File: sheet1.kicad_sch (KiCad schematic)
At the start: 18 parts, among them U1 8284A, U2 LS245, U22 74LS04, U25 8259A, U3 8088, U4 8087, U5 LS373, U6 LS244, U7 LS373, U8 8288, Y1 14.31818MHz

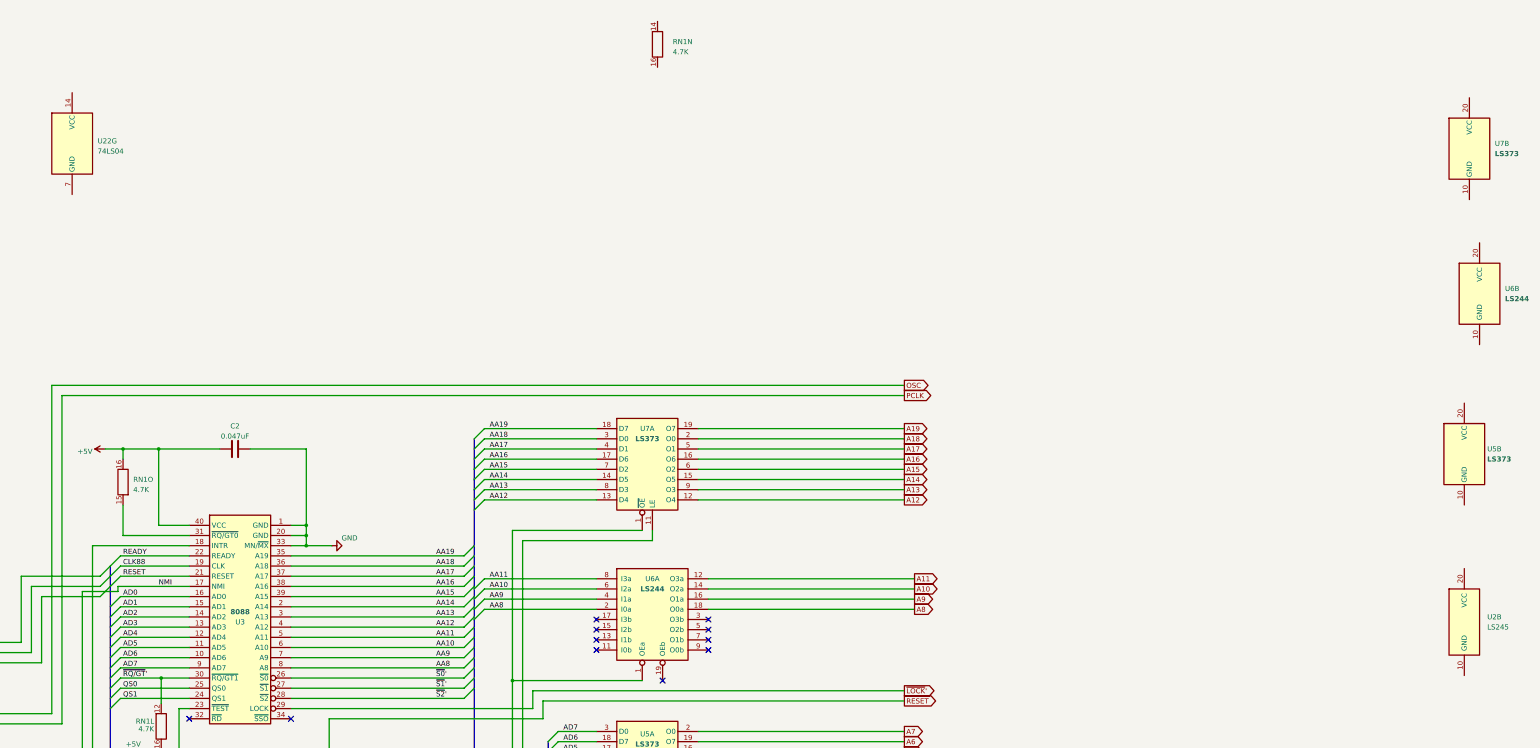
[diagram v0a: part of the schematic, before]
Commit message: Sheet 3 finished
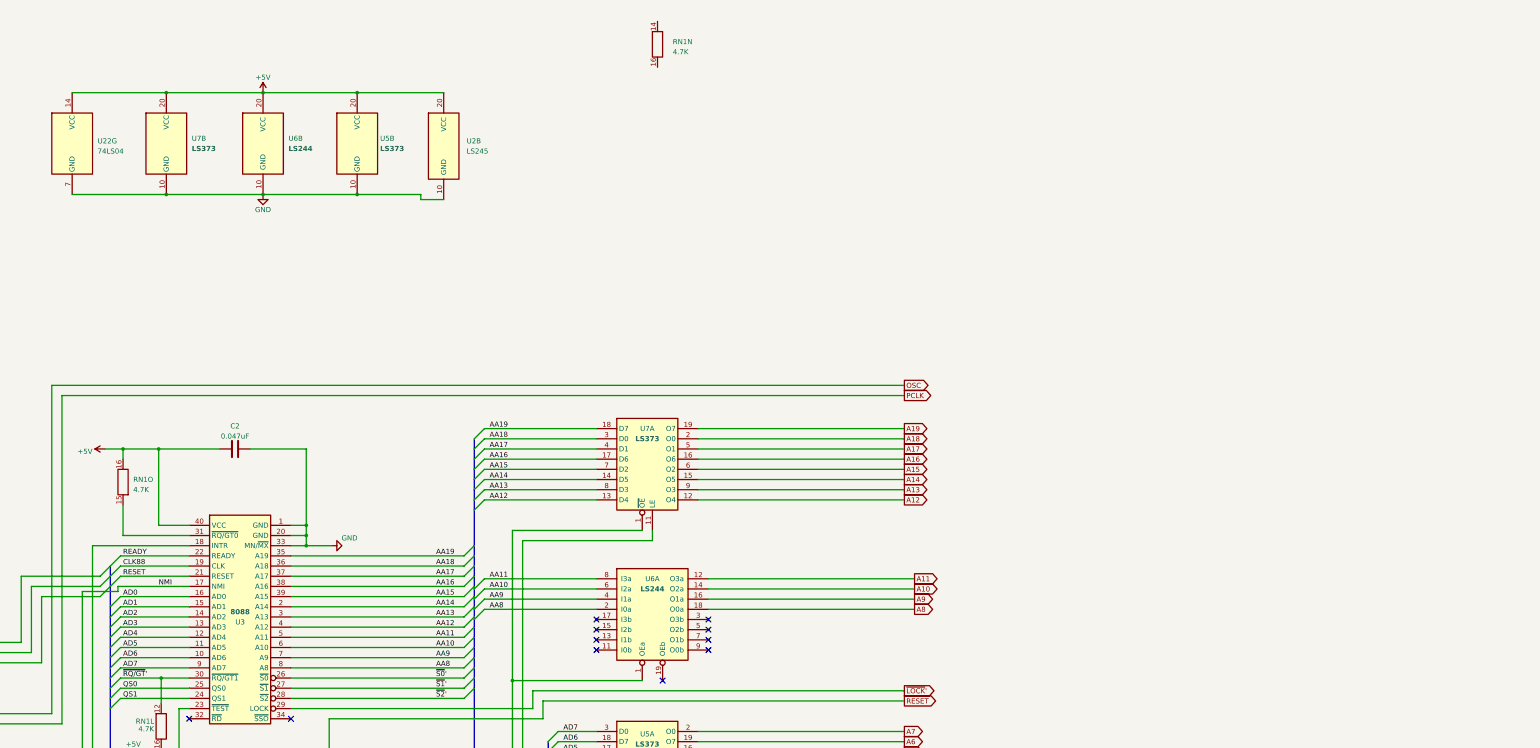
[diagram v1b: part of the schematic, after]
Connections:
- net +5V: now also U2.20 (VCC), U22.14 (VCC), U5.20 (VCC), U6.20 (VCC), U7.20 (VCC)
- net GND: now also U2.10 (GND), U22.7 (GND), U5.10 (GND), U6.10 (GND), U7.10 (GND)
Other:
- moved on the sheet: U2B, U5B, U6B, U7B
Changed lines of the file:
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@@
   (junction (at 195.58 152.4) (diameter 0) (color 0 0 0 0)
   )
+  (junction (at 183.515 -11.43) (diameter 0) (color 0 0 0 0)
+  )
   (junction (at 158.115 109.22) (diameter 0) (color 0 0 0 0)
   )
@@
   (junction (at 329.565 217.17) (diameter 0) (color 0 0 0 0)
   )
+  (junction (at 159.385 -11.43) (diameter 0) (color 0 0 0 0)
+  )
   (junction (at 321.31 214.63) (diameter 0) (color 0 0 0 0)
   )
+  (junction (at 207.01 -11.43) (diameter 0) (color 0 0 0 0)
+  )
   (junction (at 194.31 71.12) (diameter 0) (color 0 0 0 0)
   )
   (junction (at 337.82 200.66) (diameter 0) (color 0 0 0 0)
   )
+  (junction (at 207.01 -36.83) (diameter 0) (color 0 0 0 0)
+  )
   (junction (at 145.415 135.255) (diameter 0) (color 0 0 0 0)
   )
+  (junction (at 159.385 -36.83) (diameter 0) (color 0 0 0 0)
+  )
+  (junction (at 183.515 -36.83) (diameter 0) (color 0 0 0 0)
+  )
   (junction (at 247.015 242.57) (diameter 0) (color 0 0 0 0)
   )
@@
     (stroke (width 0) (type default))
   )
+  (wire (pts (xy 207.01 -11.43) (xy 222.885 -11.43))
+    (stroke (width 0) (type default))
+  )
   (wire (pts (xy 164.465 157.48) (xy 160.02 157.48))
     (stroke (width 0) (type default))
@@
     (stroke (width 0) (type default))
   )
+  (wire (pts (xy 159.385 -36.83) (xy 183.515 -36.83))
+    (stroke (width 0) (type default))
+  )
   (wire (pts (xy 297.18 191.77) (xy 297.18 203.2))
     (stroke (width 0) (type default))
@@
     (stroke (width 0) (type default))
   )
+  (wire (pts (xy 135.89 -36.83) (xy 159.385 -36.83))
+    (stroke (width 0) (type default))
+  )
   (wire (pts (xy 128.27 88.9) (xy 142.875 88.9))
     (stroke (width 0) (type default))
@@
     (stroke (width 0) (type default))
   )
+  (wire (pts (xy 183.515 -11.43) (xy 207.01 -11.43))
+    (stroke (width 0) (type default))
+  )
   (bus (pts (xy 236.22 182.88) (xy 236.22 185.42))
     (stroke (width 1) (type default) (color 0 132 0 1))
@@
     (stroke (width 0) (type default))
   )
+  (wire (pts (xy 183.515 -36.83) (xy 207.01 -36.83))
+    (stroke (width 0) (type default))
+  )
   (wire (pts (xy 147.955 109.22) (xy 158.115 109.22))
     (stroke (width 0) (type default))
@@
     (stroke (width 0) (type default))
   )
+  (wire (pts (xy 222.885 -10.16) (xy 228.6 -10.16))
+    (stroke (width 0) (type default))
+  )
   (wire (pts (xy 147.955 175.26) (xy 164.465 175.26))
     (stroke (width 0) (type default))
@@
     (stroke (width 0) (type default))
   )
+  (wire (pts (xy 222.885 -11.43) (xy 222.885 -10.16))
+    (stroke (width 0) (type default))
+  )
   (wire (pts (xy 346.075 200.66) (xy 354.33 200.66))
     (stroke (width 0) (type default))
@@
     (stroke (width 0) (type default))
   )
+  (wire (pts (xy 135.89 -11.43) (xy 159.385 -11.43))
+    (stroke (width 0) (type default))
+  )
+  (wire (pts (xy 159.385 -11.43) (xy 183.515 -11.43))
+    (stroke (width 0) (type default))
+  )
   (wire (pts (xy 147.955 83.82) (xy 165.1 83.82))
     (stroke (width 0) (type default))
@@
     (stroke (width 0) (type default))
   )
+  (wire (pts (xy 207.01 -36.83) (xy 228.6 -36.83))
+    (stroke (width 0) (type default))
+  )
   (bus (pts (xy 236.22 62.23) (xy 236.22 64.77))
     (stroke (width 1) (type default) (color 0 132 0 1))
@@
     )
   )
-  (symbol (lib_id "Mad5150_early:LS245_U2") (at 483.235 95.885 0) (unit 2)
+  (symbol (lib_id "Mad5150_early:LS245_U2") (at 228.6 -22.86 0) (unit 2)
     (in_bom yes) (on_board yes) (dnp no) (fields_autoplaced)
-    (property "Reference" "U2" (at 488.95 93.98 0)
+    (property "Reference" "U2" (at 234.315 -24.765 0)
       (effects (font (size 1.27 1.27)) (justify left))
     )
-    (property "Value" "LS245" (at 488.95 96.52 0)
+    (property "Value" "LS245" (at 234.315 -22.225 0)
       (effects (font (size 1.27 1.27)) (justify left))
     )
-    (property "Footprint" "Package_DIP:DIP-20_W7.62mm" (at 483.235 99.695 0)
+    (property "Footprint" "Package_DIP:DIP-20_W7.62mm" (at 228.6 -19.05 0)
       (effects (font (size 1.27 1.27)) hide)
     )
-    (property "Datasheet" "http://www.ti.com/lit/gpn/sn74LS245" (at 484.505 112.395 0)
+    (property "Datasheet" "http://www.ti.com/lit/gpn/sn74LS245" (at 229.87 -6.35 0)
       (effects (font (size 1.27 1.27)) hide)
     )
@@
     )
   )
+  (symbol (lib_id "power:GND") (at 183.515 -11.43 0) (unit 1)
+    (in_bom yes) (on_board yes) (dnp no)
+    (property "Reference" "#PWR033" (at 183.515 -5.08 0)
+      (effects (font (size 1.27 1.27)) hide)
+    )
+    (property "Value" "GND" (at 183.515 -7.62 0)
+      (effects (font (size 1.27 1.27)))
+    )
+    (property "Footprint" "" (at 183.515 -11.43 0)
+      (effects (font (size 1.27 1.27)) hide)
+    )
+    (property "Datasheet" "" (at 183.515 -11.43 0)
+      (effects (font (size 1.27 1.27)) hide)
+    )
+    (pin "1")
+    (instances
+      (project "Mad5160"
+        (path "/ac3c86ab-084e-42f6-87ca-c4b0142d8ff2/921209e9-21b1-4dfe-a217-0f57a16b1ecc"
+          (reference "#PWR033") (unit 1)
+        )
+      )
+    )
+  )
   (symbol (lib_id "Mad5150_early:Resistor_Network") (at -81.915 135.89 0) (unit 5)
     (in_bom yes) (on_board yes) (dnp no) (fields_autoplaced)
@@
     )
   )
-  (symbol (lib_id "Mad5150_early:LS244_U6") (at 487.045 13.335 0) (unit 2)
+  (symbol (lib_id "Mad5150_early:LS244_U6") (at 183.515 -24.13 0) (unit 2)
     (in_bom yes) (on_board yes) (dnp no) (fields_autoplaced)
-    (property "Reference" "U6" (at 493.395 12.065 0)
+    (property "Reference" "U6" (at 189.865 -25.4 0)
       (effects (font (size 1.27 1.27)) (justify left))
     )
-    (property "Value" "LS244" (at 493.395 14.605 0)
+    (property "Value" "LS244" (at 189.865 -22.86 0)
       (effects (font (size 1.27 1.27) bold) (justify left))
     )
-    (property "Footprint" "Package_DIP:DIP-20_W7.62mm" (at 487.045 13.335 0)
+    (property "Footprint" "Package_DIP:DIP-20_W7.62mm" (at 183.515 -24.13 0)
       (effects (font (size 1.27 1.27)) hide)
     )
-    (property "Datasheet" "http://www.ti.com/lit/ds/symlink/sn74ls244.pdf" (at 488.315 28.575 0)
+    (property "Datasheet" "http://www.ti.com/lit/ds/symlink/sn74ls244.pdf" (at 184.785 -8.89 0)
       (effects (font (size 1.27 1.27)) hide)
     )
@@
     )
   )
-  (symbol (lib_id "Mad5150_early:LS373_U7") (at 484.505 -22.86 0) (unit 2)
+  (symbol (lib_id "Mad5150_early:LS373_U7") (at 159.385 -24.13 0) (unit 2)
     (in_bom yes) (on_board yes) (dnp no) (fields_autoplaced)
-    (property "Reference" "U7" (at 490.855 -24.13 0)
+    (property "Reference" "U7" (at 165.735 -25.4 0)
       (effects (font (size 1.27 1.27)) (justify left))
     )
-    (property "Value" "LS373" (at 490.855 -21.59 0)
+    (property "Value" "LS373" (at 165.735 -22.86 0)
       (effects (font (size 1.27 1.27) bold) (justify left))
     )
-    (property "Footprint" "Package_DIP:DIP-20_W7.62mm" (at 484.505 -19.05 0)
+    (property "Footprint" "Package_DIP:DIP-20_W7.62mm" (at 159.385 -20.32 0)
       (effects (font (size 1.27 1.27)) hide)
     )
-    (property "Datasheet" "http://www.ti.com/lit/gpn/sn74LS373" (at 485.775 -8.89 0)
+    (property "Datasheet" "http://www.ti.com/lit/gpn/sn74LS373" (at 160.655 -10.16 0)
       (effects (font (size 1.27 1.27)) hide)
     )
@@
     )
   )
+  (symbol (lib_id "power:+5V") (at 183.515 -36.83 0) (unit 1)
+    (in_bom yes) (on_board yes) (dnp no)
+    (property "Reference" "#PWR032" (at 183.515 -33.02 0)
+      (effects (font (size 1.27 1.27)) hide)
+    )
+    (property "Value" "+5V" (at 183.515 -40.64 0)
+      (effects (font (size 1.27 1.27)))
+    )
+    (property "Footprint" "" (at 183.515 -36.83 0)
+      (effects (font (size 1.27 1.27)) hide)
+    )
+    (property "Datasheet" "" (at 183.515 -36.83 0)
+      (effects (font (size 1.27 1.27)) hide)
+    )
+    (pin "1")
+    (instances
+      (project "Mad5160"
+        (path "/ac3c86ab-084e-42f6-87ca-c4b0142d8ff2/921209e9-21b1-4dfe-a217-0f57a16b1ecc"
+          (reference "#PWR032") (unit 1)
+        )
+      )
+    )
+  )
   (symbol (lib_id "Device:Crystal") (at 108.585 91.44 90) (unit 1)
     (in_bom yes) (on_board yes) (dnp no)
@@
     )
   )
-  (symbol (lib_id "Mad5150_early:LS373_U5") (at 483.235 53.34 0) (unit 2)
+  (symbol (lib_id "Mad5150_early:LS373_U5") (at 207.01 -24.13 0) (unit 2)
     (in_bom yes) (on_board yes) (dnp no) (fields_autoplaced)
-    (property "Reference" "U5" (at 488.95 52.07 0)
+    (property "Reference" "U5" (at 212.725 -25.4 0)
       (effects (font (size 1.27 1.27)) (justify left))
     )
-    (property "Value" "LS373" (at 488.95 54.61 0)
+    (property "Value" "LS373" (at 212.725 -22.86 0)
       (effects (font (size 1.27 1.27) bold) (justify left))
     )
-    (property "Footprint" "Package_DIP:DIP-20_W7.62mm" (at 483.235 57.15 0)
+    (property "Footprint" "Package_DIP:DIP-20_W7.62mm" (at 207.01 -20.32 0)
       (effects (font (size 1.27 1.27)) hide)
     )
-    (property "Datasheet" "http://www.ti.com/lit/gpn/sn74LS373" (at 484.505 67.31 0)
+    (property "Datasheet" "http://www.ti.com/lit/gpn/sn74LS373" (at 208.28 -10.16 0)
       (effects (font (size 1.27 1.27)) hide)
     )
